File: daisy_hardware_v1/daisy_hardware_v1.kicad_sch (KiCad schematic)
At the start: 48 parts, among them J1 Conn_02x08_Odd_Even, J2 PJ398SM-12, J20 Conn_01x18_Female, J21 Conn_01x18_Female, J3 PJ398SM-12, J4 PJ398SM-12, J5 PJ398SM-12, J6 Conn_01x18_Male, J9 Conn_01x18_Male, SW1 SW_SPDT, SW2 SW_SPDT, U1 RAF_DAISY_SEED_V1, U10 LM1117-5.0, U11 TL072, U2 TL072, U3 74HC4051, U4 74HC4051, U5 LM4040DBZ-10, U6 MCP6004, U7 MCP6004, U8 MCP6002-xSN, U9 R-78E3.3-0.5

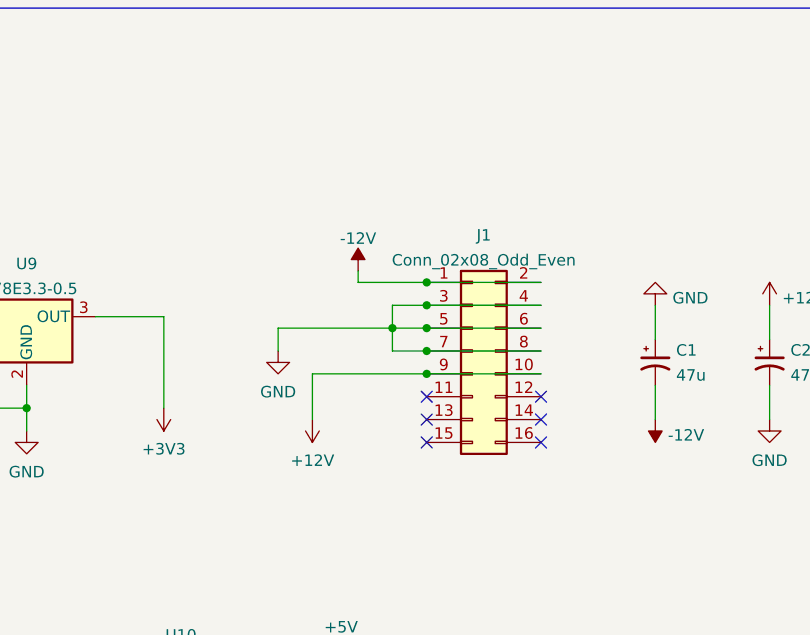
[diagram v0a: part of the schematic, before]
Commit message: another export
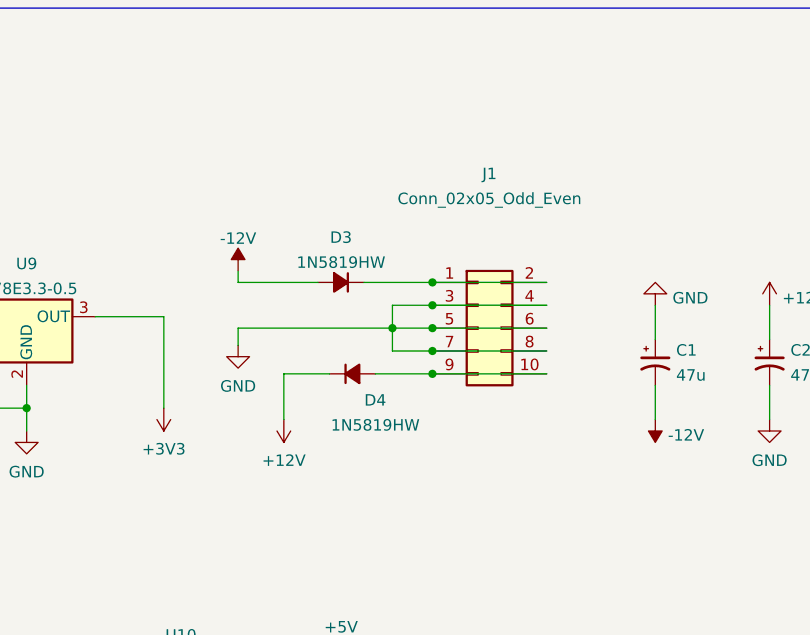
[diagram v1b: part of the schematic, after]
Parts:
- removed J1: Conn_02x08_Odd_Even, Connector_PinHeader_2.54mm:PinHeader_2x08_P2.54mm_Vertical, symbol Connector_Generic:Conn_02x08_Odd_Even
- added D3, D4: 1N5819HW, Diode_SMD:D_SOD-123, symbol Device:D_Small_Filled
- added J1: Conn_02x05_Odd_Even, Connector_PinHeader_2.54mm:PinHeader_2x05_P2.54mm_Vertical, symbol Connector_Generic:Conn_02x05_Odd_Even
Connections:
- net +12V: now also D4.1 (K)
- net -12V: now also D3.2 (A)
- net GND: now also J1.3 (Pin_3), J1.4 (Pin_4), J1.5 (Pin_5), J1.6 (Pin_6), J1.7 (Pin_7), J1.8 (Pin_8)
- new net: D3.1 (K), J1.1 (Pin_1), J1.2 (Pin_2)
- new net: D4.2 (A), J1.10 (Pin_10), J1.9 (Pin_9)
- no-connect marks 16 -> 10
